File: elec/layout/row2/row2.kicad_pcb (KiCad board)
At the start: 2 copper layers, 10 parts

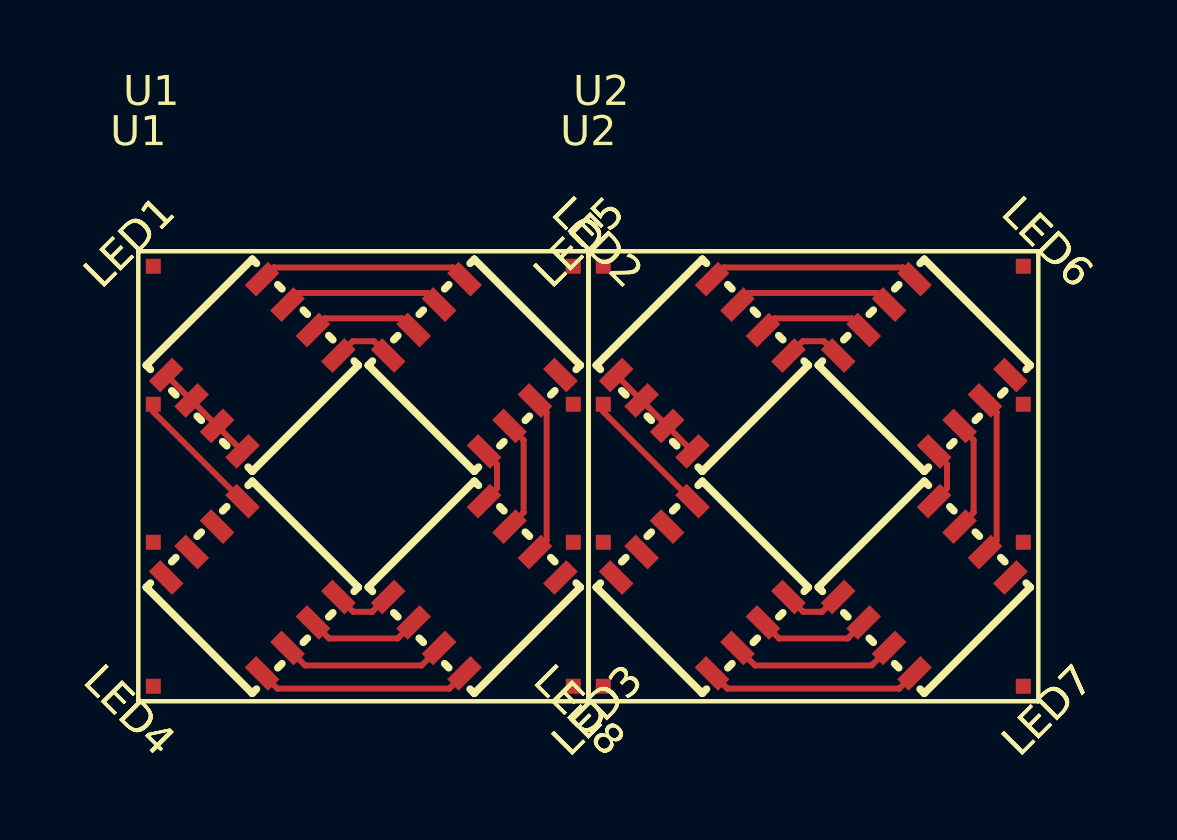
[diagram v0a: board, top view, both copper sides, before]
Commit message: updating rp2040
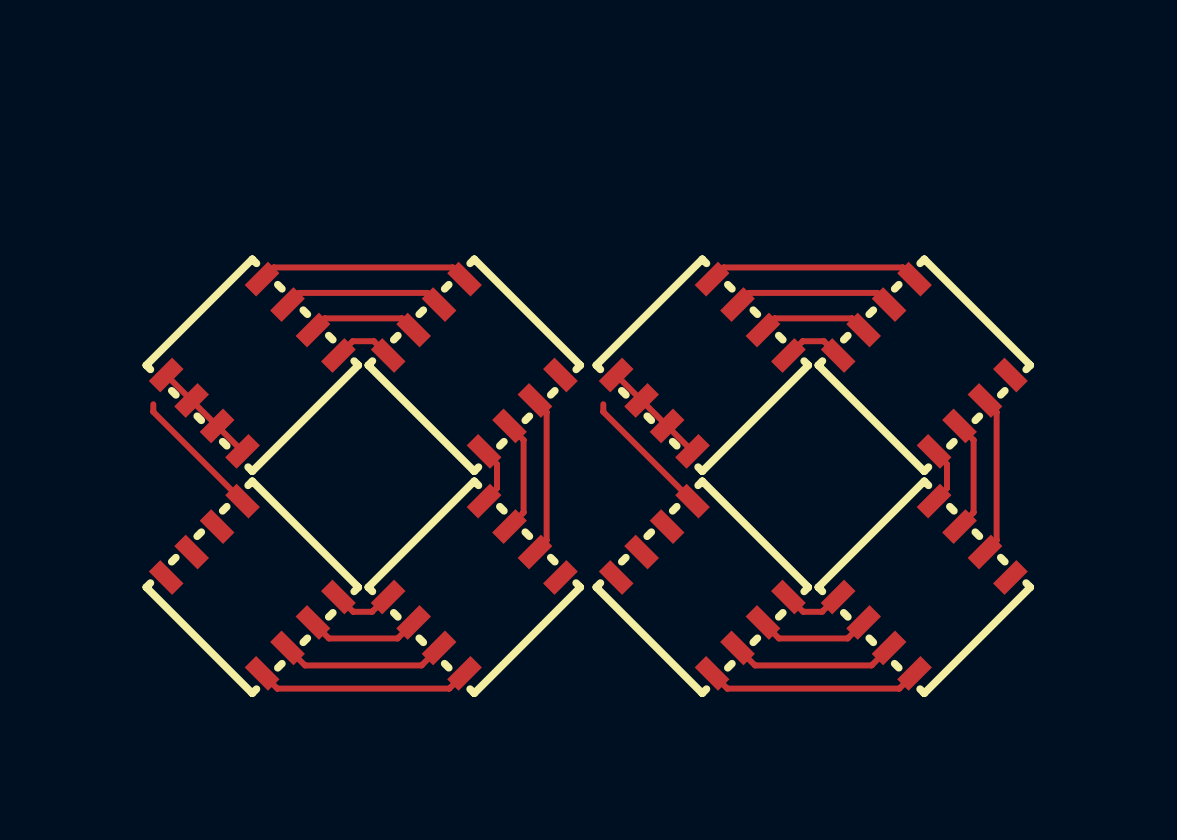
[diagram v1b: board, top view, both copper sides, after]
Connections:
- net pixels[0]-blue-1 renamed rgbs[1]-anodes-anode-0
- net pixels[0]-blue-2 renamed rgbs[2]-anodes-anode-0
- net pixels[0]-blue-3 renamed rgbs[3]-anodes-anode-0
- net pixels[0]-cold_white-1 renamed rgbs[1]-anodes-anode-1
- net pixels[0]-cold_white-2 renamed rgbs[2]-anodes-anode-1
- net pixels[0]-cold_white-3 renamed rgbs[3]-anodes-anode-1
- net pixels[0]-green-1 renamed rgbs[1]-anodes-anode-2
- net pixels[0]-green-2 renamed rgbs[2]-anodes-anode-2
- net pixels[0]-green-3 renamed rgbs[3]-anodes-anode-2
- net pixels[0]-red-1 renamed rgbs[1]-anodes-anode-3
- net pixels[0]-red-2 renamed rgbs[2]-anodes-anode-3
- net pixels[0]-red-3 renamed rgbs[3]-anodes-anode-3
- net pixels[1]-blue-1 renamed rgbs[1]-anodes-anode-4
- net pixels[1]-blue-2 renamed rgbs[2]-anodes-anode-4
- net pixels[1]-blue-3 renamed rgbs[3]-anodes-anode-4
- net pixels[1]-cold_white-1 renamed rgbs[1]-anodes-anode-5
- net pixels[1]-cold_white-2 renamed rgbs[2]-anodes-anode-5
- net pixels[1]-cold_white-3 renamed rgbs[3]-anodes-anode-5
- net pixels[1]-green-1 renamed rgbs[1]-anodes-anode-6
- net pixels[1]-green-2 renamed rgbs[2]-anodes-anode-6
- net pixels[1]-green-3 renamed rgbs[3]-anodes-anode-6
- net pixels[1]-red-1 renamed rgbs[1]-anodes-anode-7
- net pixels[1]-red-2 renamed rgbs[2]-anodes-anode-7
- net pixels[1]-red-3 renamed rgbs[3]-anodes-anode-7
- LED1 pad 2: pixels[0]-anode -> rgbs[0]-anodes-anode-0
- LED1 pad 4: pixels[0]-anode -> rgbs[0]-anodes-anode-0
- LED1 pad 6: pixels[0]-anode -> rgbs[0]-anodes-anode-0
- LED1 pad 8: pixels[0]-anode -> rgbs[0]-anodes-anode-0
- LED4 pad 1: pixels[0]-cold_white-0 -> rgbs[3]-cathodes-cathode-1
- LED4 pad 3: pixels[0]-blue-0 -> rgbs[3]-cathodes-cathode-0
- LED4 pad 5: pixels[0]-green-0 -> rgbs[3]-cathodes-cathode-2
- LED4 pad 7: pixels[0]-red-0 -> rgbs[3]-cathodes-cathode-3
- LED5 pad 2: pixels[1]-anode -> rgbs[0]-anodes-anode-1
- LED5 pad 4: pixels[1]-anode -> rgbs[0]-anodes-anode-1
- LED5 pad 6: pixels[1]-anode -> rgbs[0]-anodes-anode-1
- LED5 pad 8: pixels[1]-anode -> rgbs[0]-anodes-anode-1
- LED8 pad 1: pixels[1]-cold_white-0 -> rgbs[3]-cathodes-cathode-5
- LED8 pad 3: pixels[1]-blue-0 -> rgbs[3]-cathodes-cathode-4
- LED8 pad 5: pixels[1]-green-0 -> rgbs[3]-cathodes-cathode-6
- LED8 pad 7: pixels[1]-red-0 -> rgbs[3]-cathodes-cathode-7
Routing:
- net rgbs[3]-cathodes-cathode-7: track 0.00 -> 4.46 mm
- net rgbs[3]-cathodes-cathode-3: track 0.00 -> 4.46 mm
- net pixels[1]-red-0: track 4.46 -> 0.00 mm
- net pixels[0]-red-0: track 4.46 -> 0.00 mm
- net rgbs[0]-anodes-anode-0: track 0.00 -> 3.60 mm
- net pixels[0]-anode: track 3.60 -> 0.00 mm
- net rgbs[0]-anodes-anode-1: track 0.00 -> 3.60 mm
- net pixels[1]-anode: track 3.60 -> 0.00 mm

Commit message: tight layout
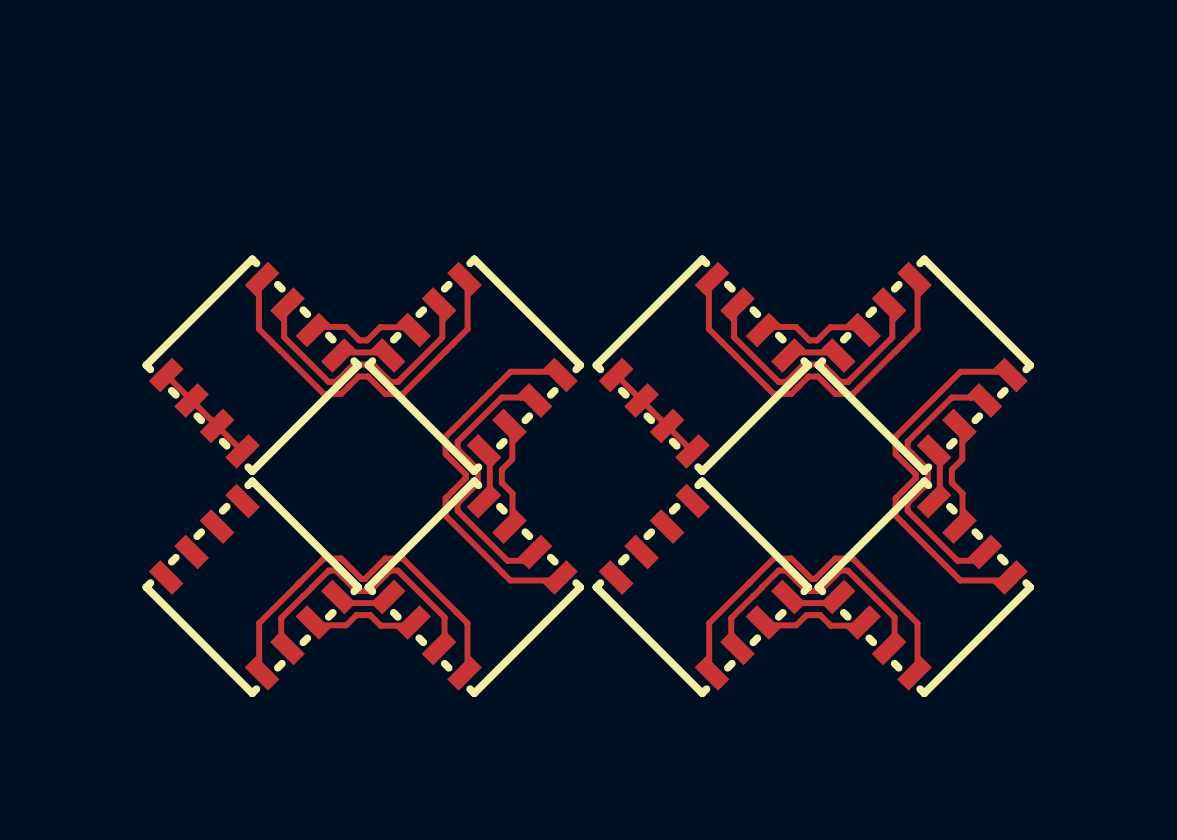
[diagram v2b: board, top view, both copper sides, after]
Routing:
- net rgbs[2]-anodes-anode-5: track 0.00 -> 12.3 mm
- net rgbs[2]-anodes-anode-1: track 0.00 -> 12.3 mm
- net rgbs[3]-anodes-anode-5: track 7.17 -> 12.8 mm
- net rgbs[3]-anodes-anode-1: track 7.17 -> 12.8 mm
- net rgbs[1]-anodes-anode-5: track 7.07 -> 12.6 mm
- net rgbs[1]-anodes-anode-1: track 7.07 -> 12.6 mm
- net rgbs[3]-cathodes-cathode-7: track 4.46 -> 0.00 mm
- net rgbs[3]-cathodes-cathode-3: track 4.46 -> 0.00 mm
- net rgbs[2]-anodes-anode-4: track 5.37 -> 9.48 mm
- net rgbs[2]-anodes-anode-0: track 5.37 -> 9.48 mm
- net rgbs[3]-anodes-anode-4: track 5.54 -> 9.49 mm
- net rgbs[3]-anodes-anode-0: track 5.54 -> 9.49 mm
- net rgbs[1]-anodes-anode-4: track 5.37 -> 9.26 mm
- net rgbs[1]-anodes-anode-0: track 5.37 -> 9.26 mm
